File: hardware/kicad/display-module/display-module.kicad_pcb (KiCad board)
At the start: 2 copper layers, 8 parts, among them J1 Exp0, U1 74LS00, U2 74LS373

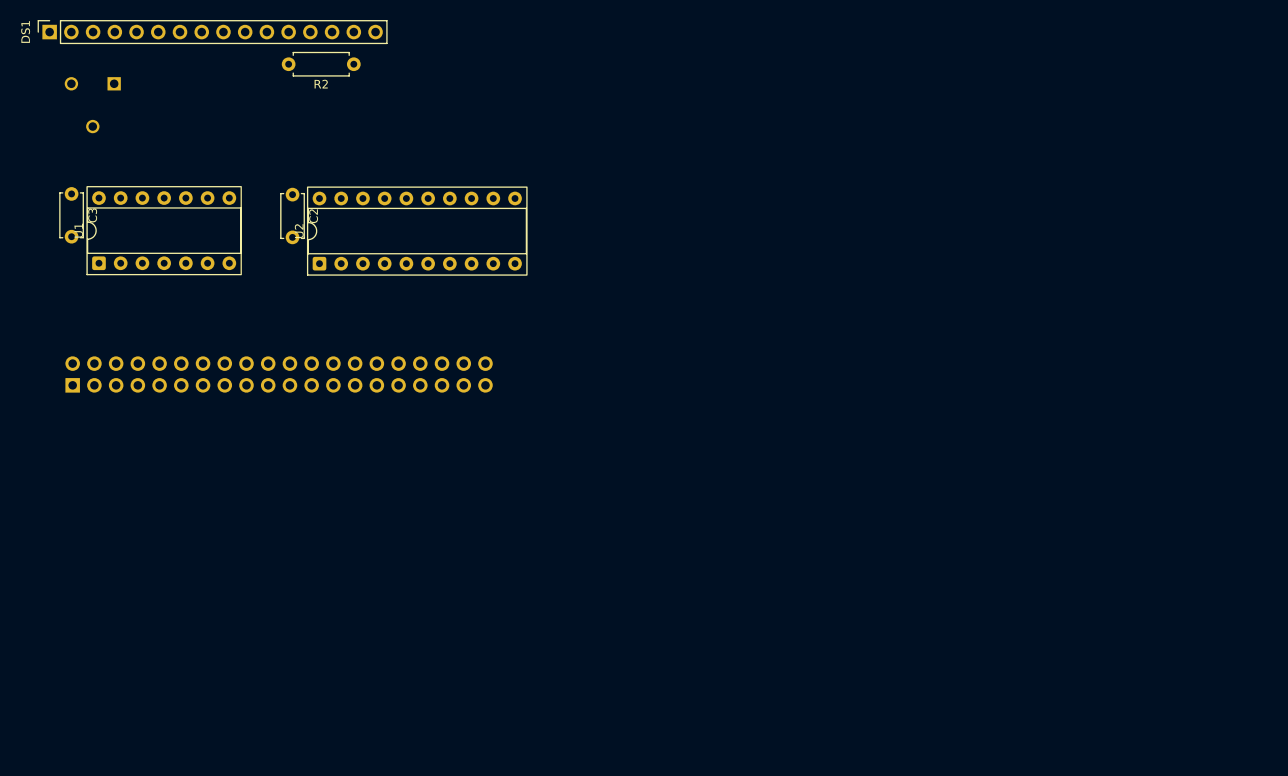
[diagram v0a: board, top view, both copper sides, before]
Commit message: Add mainboard v2.0 (#6)
* Add mainboard v2.0
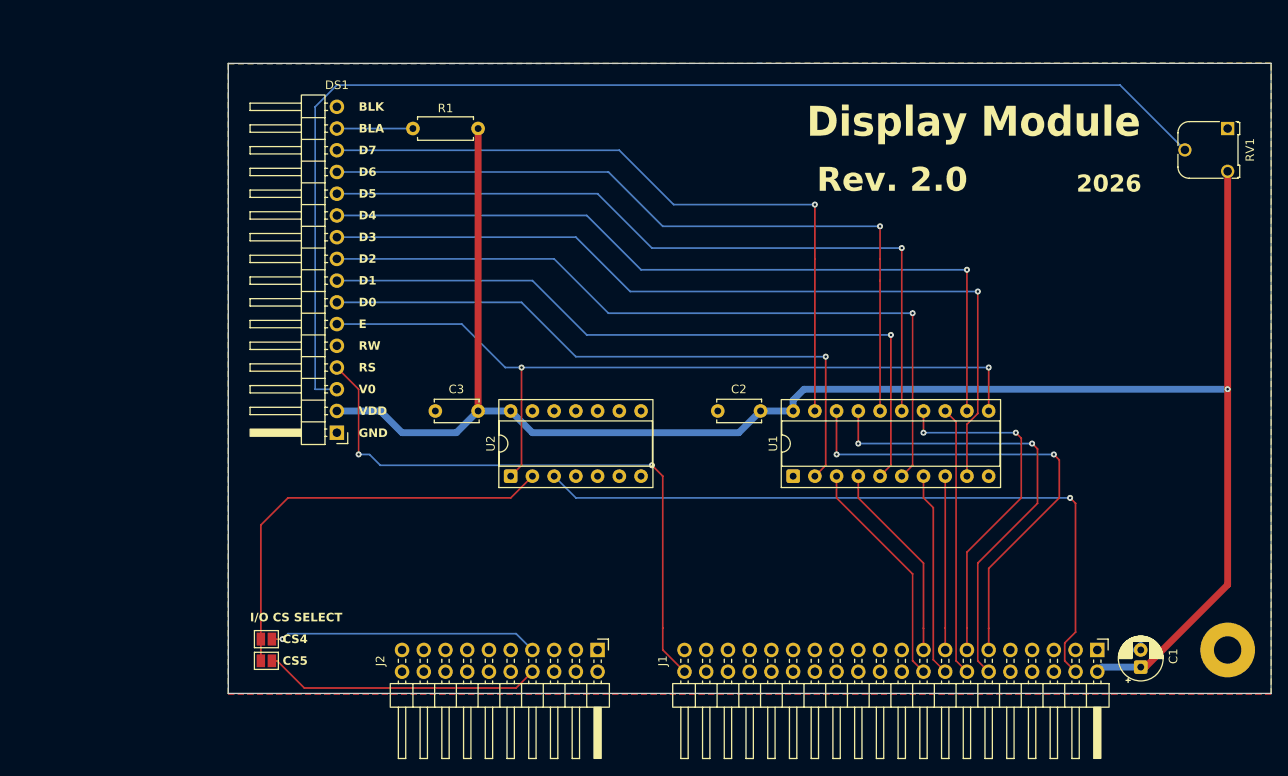
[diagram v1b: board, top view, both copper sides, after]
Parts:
- removed the U1 at (76.3, 69.1)
- added C1: 220 uF, Capacitor_THT:CP_Radial_D5.0mm_P2.00mm, F.Cu at (198.1, 116.3)
- added H1: MountingHole_Pad, MountingHole:MountingHole_3.2mm_M3_Pad, F.Cu at (208.3, 114.3)
- added J2: EXP_0_B, Connector_PinHeader_2.54mm:PinHeader_2x10_P2.54mm_Horizontal, F.Cu at (134.6, 114.3)
- added JP1: Jumper_2_Small_Open, Jumper:SolderJumper-2_P1.3mm_Open_Pad1.0x1.5mm, F.Cu at (95.9, 113.0)
- added JP2: Jumper_2_Small_Open, Jumper:SolderJumper-2_P1.3mm_Open_Pad1.0x1.5mm, F.Cu at (95.9, 115.6)
- added U2: 74LS02, Package_DIP:DIP-14_W7.62mm_Socket, F.Cu at (124.5, 94.0)
- DS1: value WC1602A -> WC1604A; footprint Connector_PinSocket_2.54mm:PinSocket_1x16_P2.54mm_Vertical -> Connector_PinHeader_2.54mm:PinHeader_1x16_P2.54mm_Horizontal
- J1: value Exp0 -> EXP_0_A; footprint Connector_PinSocket_2.54mm:PinSocket_2x20_P2.54mm_Vertical -> Connector_PinHeader_2.54mm:PinHeader_2x20_P2.54mm_Horizontal; moved to F.Cu
- RV1: moved to F.Cu
- moved RV1 130.3 mm to (208.3, 53.3), turned to -90 degrees
- moved J1 123.7 mm to (193.0, 114.3)
- moved U1 60.7 mm to (157.5, 94.0)
- moved C2 60.3 mm to (153.7, 86.4), turned to 180 degrees
- moved DS1 57.6 mm to (104.1, 88.9), turned to 180 degrees
- moved C3 53.9 mm to (120.7, 86.4), turned to 180 degrees
- moved R1 10.2 mm to (113.0, 53.3), turned to 0 degrees
- renumbered R2 to R1, U2 to U1
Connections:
- J1 pad 10: /A12 -> GND
- J1 pad 11: /A11 -> /D7
- J1 pad 12: /A10 -> /D6
- J1 pad 13: /A9 -> /D5
- J1 pad 14: /A8 -> /D4
- J1 pad 15: /A7 -> /D3
- J1 pad 16: /A6 -> /D2
- J1 pad 17: /A5 -> /D1
- J1 pad 18: /A4 -> /D0
- J1 pad 19: /A3 -> GND
- J1 pad 20: /A2 -> GND
- J1 pad 21: /A1 -> /A19
- J1 pad 22: /A0 -> /A18
- J1 pad 23: /D7 -> /A17
- J1 pad 24: /D6 -> /A16
- J1 pad 25: /D5 -> /A15
- J1 pad 26: /D4 -> /A14
- J1 pad 27: /D3 -> /A13
- J1 pad 28: /D2 -> /A12
- J1 pad 29: /D1 -> /A11
- J1 pad 3: /A19 -> /IOM
- J1 pad 30: /D0 -> /A10
- J1 pad 31: /IOM -> /A9
- J1 pad 32: /RD -> /A8
- J1 pad 33: /WR -> /A7
- J1 pad 34: /RDY -> /A6
- J1 pad 35: /RESET -> /A5
- J1 pad 36: /ALE -> /A4
- J1 pad 37: /MEM_EXP0_CS -> /A3
- J1 pad 38: /IO_EXP_CS -> /A2
- J1 pad 39: GND -> /A1
- J1 pad 4: /A18 -> /WR
- J1 pad 40: /CLK -> /A0
- J1 pad 5: /A17 -> /RD
- J1 pad 6: /A16 -> /RDY
- J1 pad 7: /A15 -> /RESET
- J1 pad 8: /A14 -> /NMI
- J1 pad 9: /A13 -> /ALE
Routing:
- net VCC: track 0.00 -> 211.0 mm, vias 0 -> 1
- net Net-(DS1-VO): track 0.00 -> 141.4 mm
- net Net-(DS1-D3): track 0.00 -> 99.7 mm, vias 0 -> 1
- net /LCD_WRITE: track 0.00 -> 96.6 mm, vias 0 -> 2
- net Net-(DS1-D4): track 0.00 -> 92.8 mm, vias 0 -> 1
- net Net-(DS1-D2): track 0.00 -> 89.5 mm, vias 0 -> 1
- net Net-(DS1-D5): track 0.00 -> 87.7 mm, vias 0 -> 1
- net Net-(DS1-D6): track 0.00 -> 87.7 mm, vias 0 -> 1
- net Net-(DS1-D1): track 0.00 -> 84.4 mm, vias 0 -> 1
- net /WR: track 0.00 -> 83.0 mm, vias 0 -> 1
- net Net-(DS1-D7): track 0.00 -> 82.6 mm, vias 0 -> 1
- net Net-(DS1-D0): track 0.00 -> 74.3 mm, vias 0 -> 1
- net /A0: track 0.00 -> 71.7 mm, vias 0 -> 2
- net /D7: track 0.00 -> 57.0 mm, vias 0 -> 2
- net /D6: track 0.00 -> 54.5 mm, vias 0 -> 2
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- added copper zone on B.Cu, net GND
- added copper zone on F.Cu, net GND
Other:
- board outline added: 121.9 x 73.7 mm
- board text added: "2026"
- board text added: "BLA"
- board text added: "BLK"
- board text added: "CS4"
- board text added: "CS5"
- board text added: "D0"
- board text added: "D1"
- board text added: "D2"
- board text added: "D3"
- board text added: "D4"
- board text added: "D5"
- board text added: "D6"
- board text added: "D7"
- board text added: "Display Module"
- board text added: "E"
- board text added: "GND"
- board text added: "I/O CS SELECT"
- board text added: "RS"
- board text added: "RW"
- board text added: "Rev. 2.0"
- board text added: "V0"
- board text added: "VDD"
